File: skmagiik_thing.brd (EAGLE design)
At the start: 55.9 x 64.4 mm, 15 parts, among them J1 AUDIO-JACK, J2 AUDIO-JACK

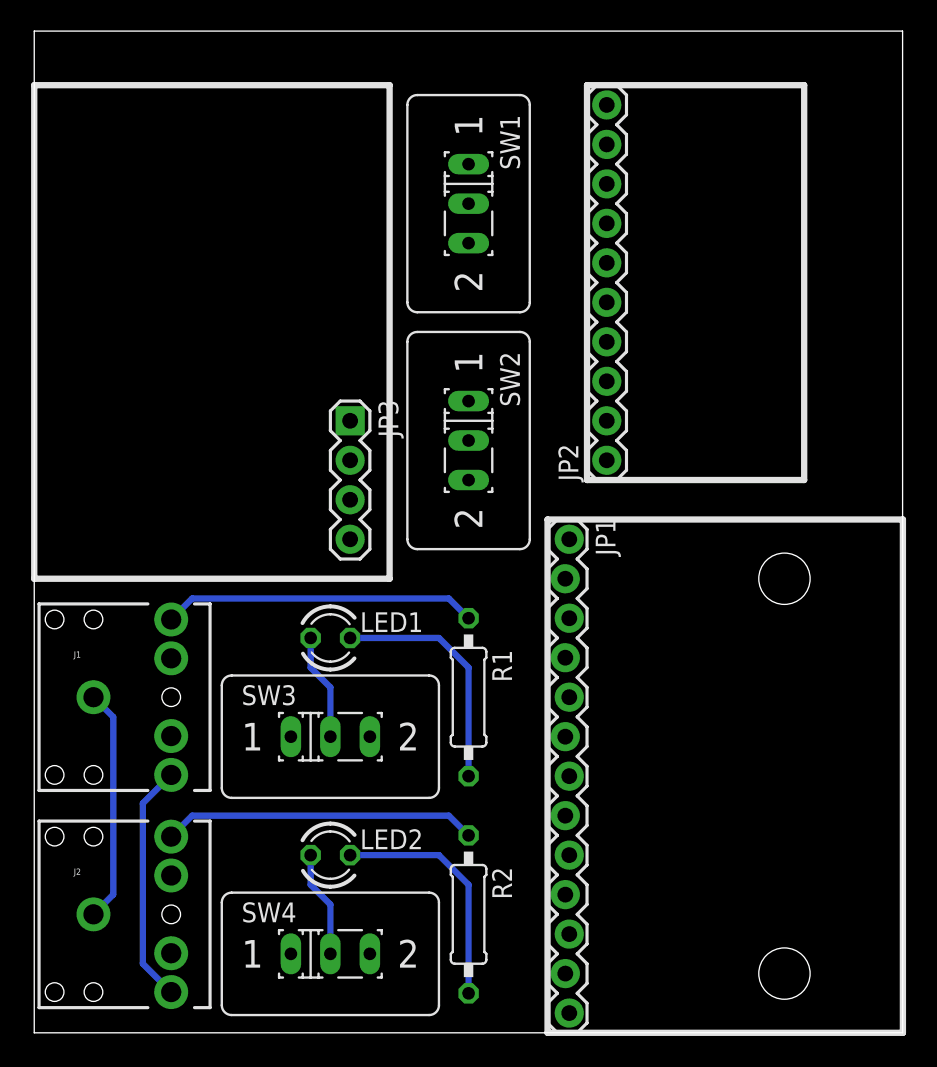
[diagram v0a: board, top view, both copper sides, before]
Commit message: layour ready for aproval
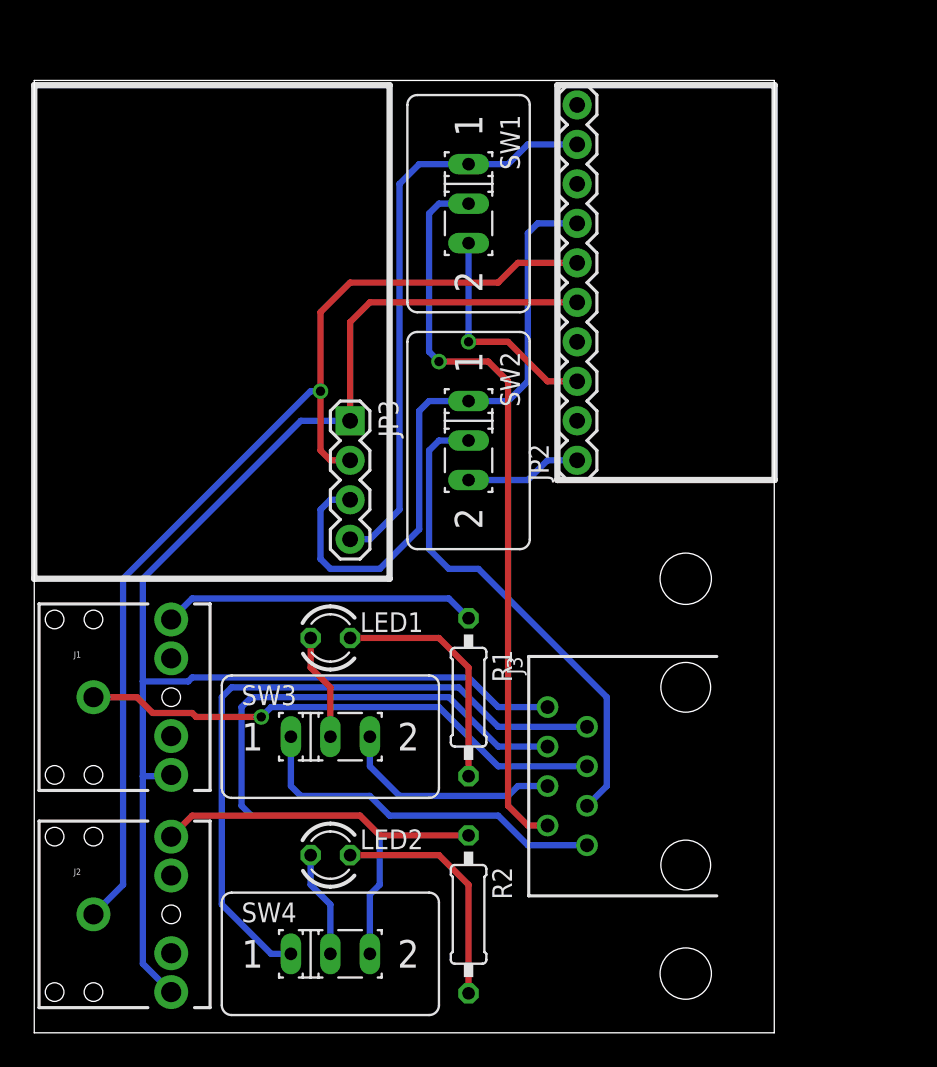
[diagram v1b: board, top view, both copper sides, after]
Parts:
- removed JP1: M13LOCK, SparkFun-Connectors:1X13_LOCK
- added J3: RJ45, pjb:RJ45
- moved STANDOFF3 6.35 mm to (41.9, 3.81)
- moved STANDOFF5 6.35 mm to (41.9, 29.2)
- moved JP2 1.91 mm to (34.9, 36.8)
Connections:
- net GND: now also J3.5; no longer JP1.9
- net N$17: now also J3.2; no longer JP1.12
- net N$18: now also J3.3; no longer JP1.11
- net N$3: now also J3.7; no longer JP1.7
- net N$4: now also J3.6; no longer JP1.8
- net N$5: now also J3.4; no longer JP1.10
- net N$6: now also J3.1; no longer JP1.13
- net VCC: now also J3.8; no longer JP1.6
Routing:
- net GND: track 15.0 -> 105.0 mm, vias 0 -> 2
- net VCC: track 15.5 -> 95.2 mm
- net N$17: track 0.00 -> 47.9 mm, vias 0 -> 1
- net N$4: track 0.00 -> 45.2 mm
- net N$3: track 0.00 -> 43.9 mm
- net N$9: track 0.00 -> 41.4 mm
- net N$11: track 0.00 -> 37.4 mm
- net N$18: track 0.00 -> 32.0 mm
- net N$6: track 0.00 -> 23.8 mm
- net N$5: track 0.00 -> 14.4 mm
- net N$13: track 0.00 -> 14.4 mm, vias 0 -> 1
- net N$10: track 0.00 -> 7.51 mm
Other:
- board size 55.9 x 64.4 mm -> 47.6 x 61.3 mm
